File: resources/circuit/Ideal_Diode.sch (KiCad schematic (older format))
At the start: 4 parts, among them Q1 BSS138, U5 DMMT5401

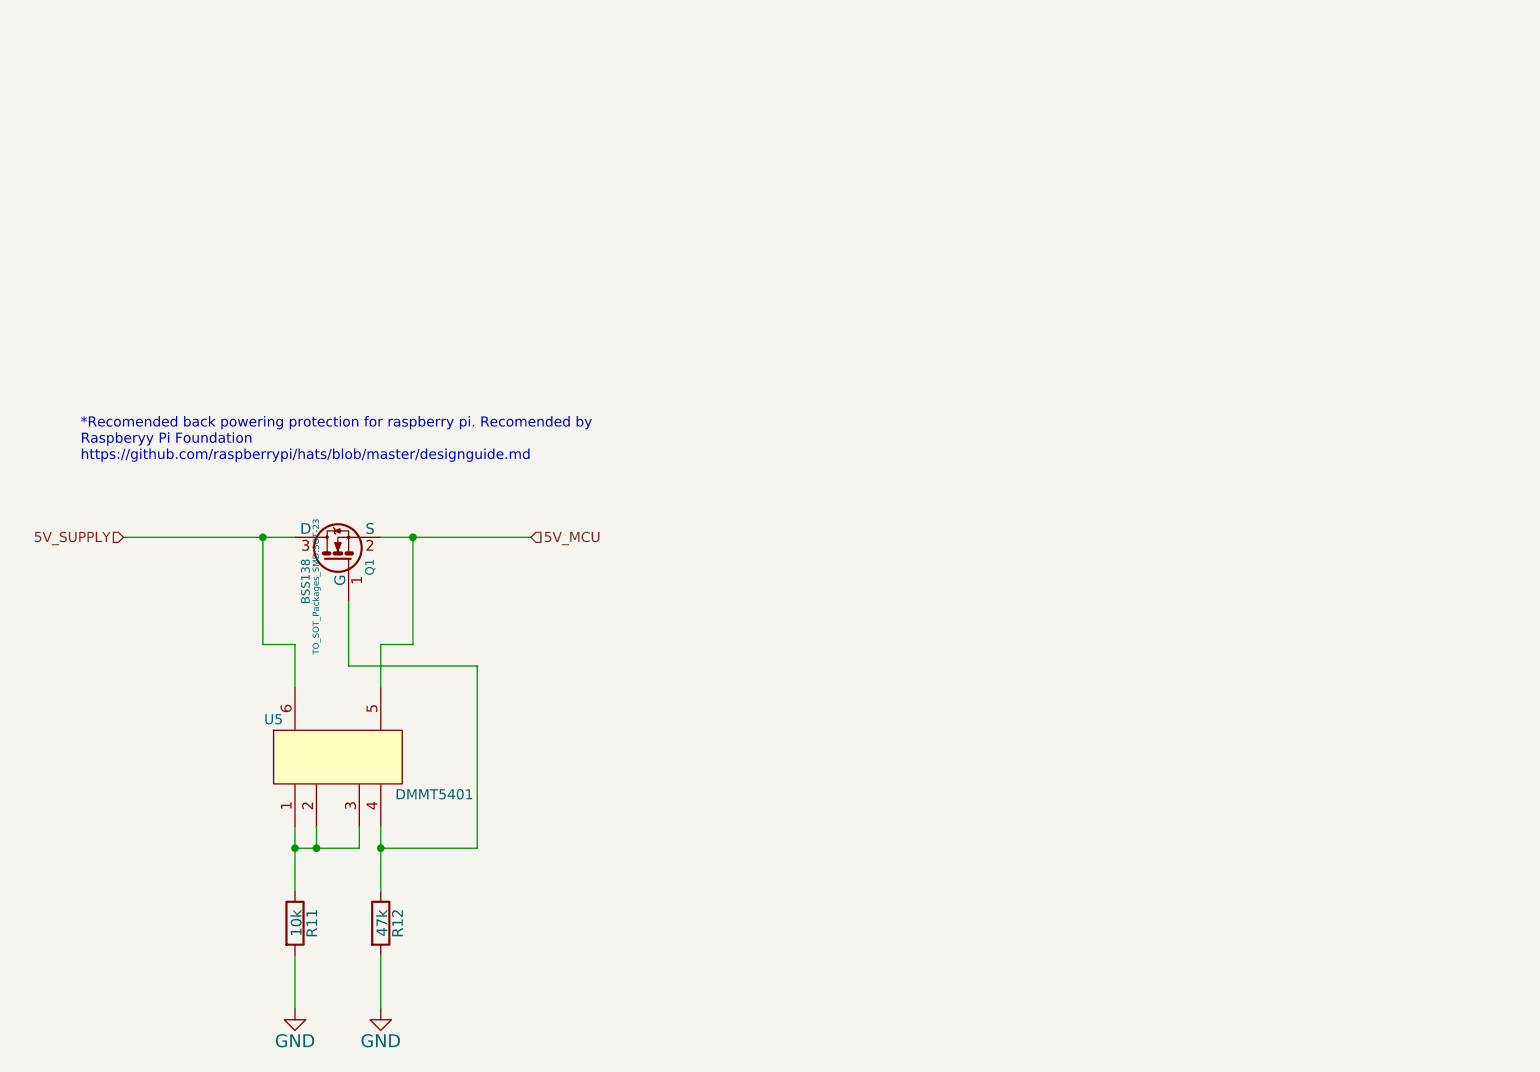
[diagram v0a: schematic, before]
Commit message: Work on circuit & PCB
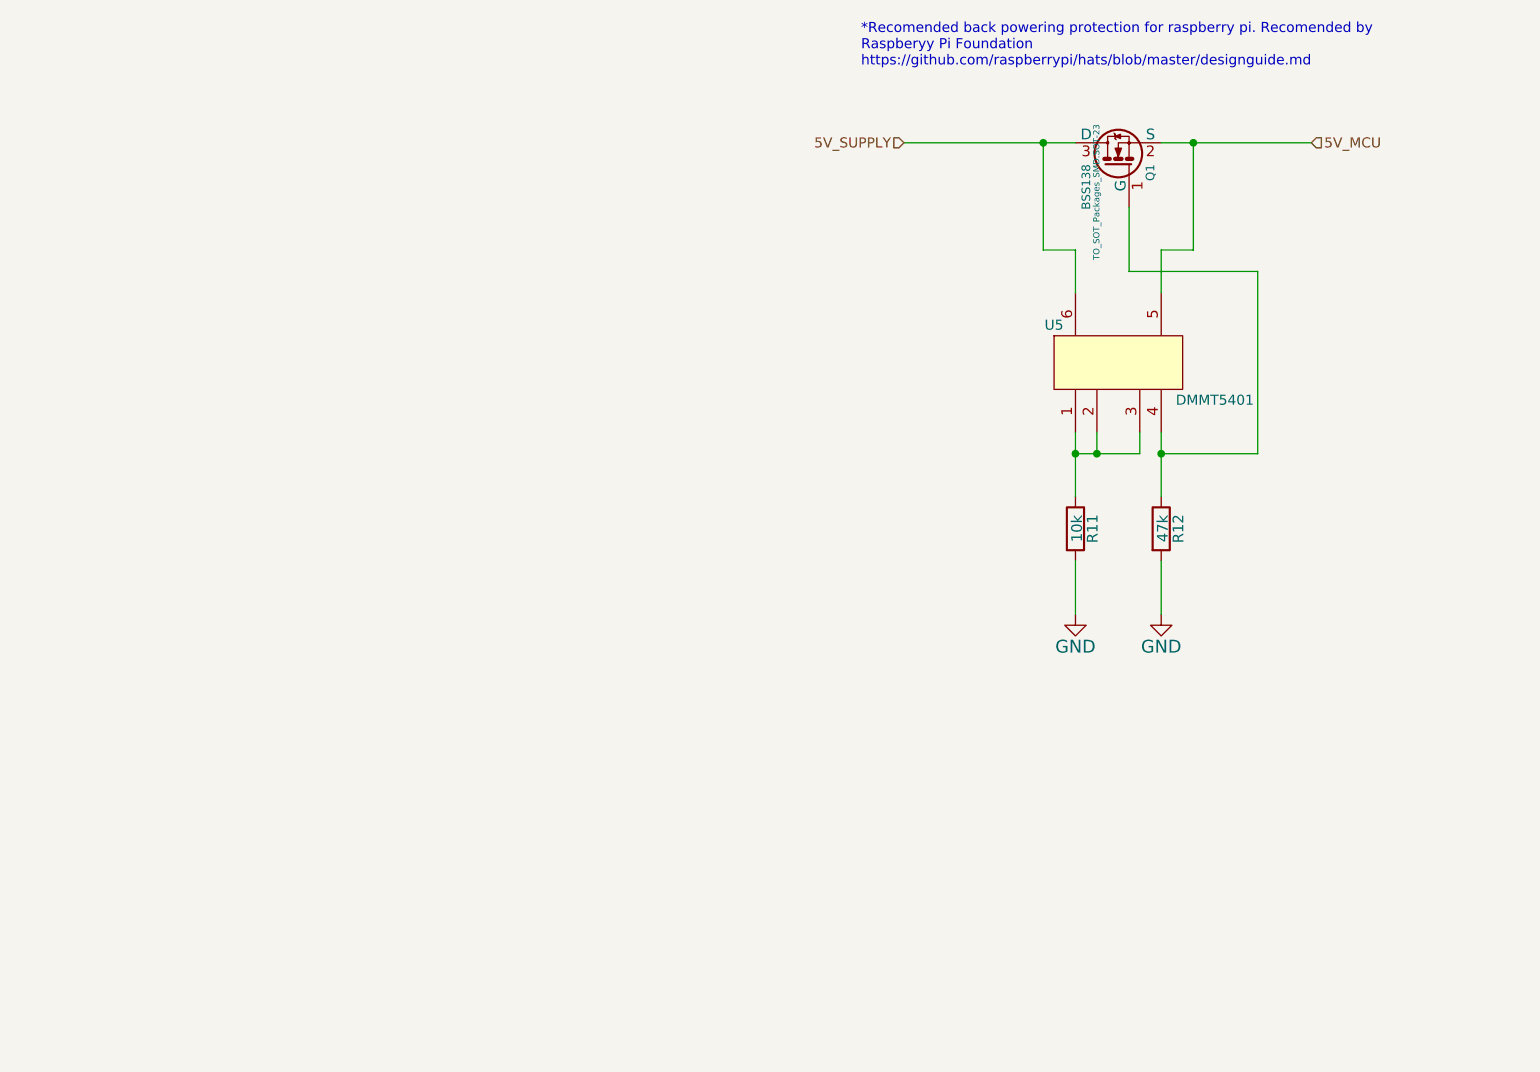
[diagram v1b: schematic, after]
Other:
- moved on the sheet: Q1, R11, R12, U5
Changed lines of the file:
@@
 LIBS:valves
 LIBS:aeroPi
+LIBS:bme280
 LIBS:aeroPi-cache
 EELAYER 25 0
@@
 $Descr A4 11693 8268
 encoding utf-8
-Sheet 2 3
+Sheet 2 2
 Title ""
 Date ""
@@
 L BSS138 Q1
 U 1 1 54F14605
-P 6000 3100
-F 0 "Q1" H 6000 2951 40  0000 R CNN
-F 1 "BSS138" H 6000 3250 40  0000 R CNN
-F 2 "TO_SOT_Packages_SMD:SOT-23" H 5870 3202 29  0000 C CNN
-F 3 "" H 6000 3100 60  0000 C CNN
-F 4 "621-DMG2305UX-13" H 6000 3100 60  0001 C CNN "Mouser Part No."
-	1    6000 3100
+P 9640 1260
+F 0 "Q1" H 9640 1111 40  0000 R CNN
+F 1 "BSS138" H 9640 1410 40  0000 R CNN
+F 2 "TO_SOT_Packages_SMD:SOT-23" H 9510 1362 29  0000 C CNN
+F 3 "" H 9640 1260 60  0000 C CNN
+F 4 "621-DMG2305UX-13" H 9640 1260 60  0001 C CNN "Mouser Part No."
+	1    9640 1260
 	0    -1   -1   0
 $EndComp
-Text HLabel 5000 3000 0    47   Input ~ 0
+Text HLabel 8640 1160 0    47   Input ~ 0
 5V_SUPPLY
-Text HLabel 6900 3000 2    47   Input ~ 0
+Text HLabel 10540 1160 2    47   Input ~ 0
 5V_MCU
 $Comp
 L DMMT5401 U5
 U 1 1 54F1CFA3
-P 6000 4000
-F 0 "U5" H 5700 4150 47  0000 C CNN
-F 1 "DMMT5401" H 6450 3800 47  0000 C CNN
-F 2 "w_smd_trans:sot23-6" H 5850 3700 47  0001 C CNN
-F 3 "" H 5850 3700 47  0000 C CNN
-F 4 "621-DMMT5401-7-F" H 6000 4000 60  0001 C CNN "Mouser Part No."
-	1    6000 4000
+P 9640 2160
+F 0 "U5" H 9340 2310 47  0000 C CNN
+F 1 "DMMT5401" H 10090 1960 47  0000 C CNN
+F 2 "w_smd_trans:sot23-6" H 9490 1860 47  0001 C CNN
+F 3 "" H 9490 1860 47  0000 C CNN
+F 4 "621-DMMT5401-7-F" H 9640 2160 60  0001 C CNN "Mouser Part No."
+	1    9640 2160
 	1    0    0    -1
 $EndComp
 Wire Wire Line
-	6200 3000 6900 3000
+	9840 1160 10540 1160
 Wire Wire Line
-	5000 3000 5800 3000
+	8640 1160 9440 1160
 Wire Wire Line
-	5800 3700 5800 3500
+	9440 1860 9440 1660
 Wire Wire Line
-	5800 3500 5650 3500
+	9440 1660 9290 1660
 Wire Wire Line
-	5650 3500 5650 3000
-Connection ~ 5650 3000
+	9290 1660 9290 1160
+Connection ~ 9290 1160
 Wire Wire Line
-	6200 3700 6200 3500
+	9840 1860 9840 1660
 Wire Wire Line
-	6200 3500 6350 3500
+	9840 1660 9990 1660
 Wire Wire Line
-	6350 3500 6350 3000
-Connection ~ 6350 3000
+	9990 1660 9990 1160
+Connection ~ 9990 1160
 $Comp
 L R R12
 U 1 1 54F1D101
-P 6200 4800
-F 0 "R12" V 6280 4800 50  0000 C CNN
-F 1 "47k" V 6207 4801 50  0000 C CNN
-F 2 "Resistors_SMD:R_0603" V 6130 4800 30  0001 C CNN
-F 3 "" H 6200 4800 30  0000 C CNN
-F 4 "667-ERJ-2RKF4702X" V 6200 4800 60  0001 C CNN "Mouser Part No."
-	1    6200 4800
+P 9840 2960
+F 0 "R12" V 9920 2960 50  0000 C CNN
+F 1 "47k" V 9847 2961 50  0000 C CNN
+F 2 "Resistors_SMD:R_0603" V 9770 2960 30  0001 C CNN
+F 3 "" H 9840 2960 30  0000 C CNN
+F 4 "667-ERJ-2RKF4702X" V 9840 2960 60  0001 C CNN "Mouser Part No."
+	1    9840 2960
 	1    0    0    -1
 $EndComp
@@
 L R R11
 U 1 1 54F1D193
-P 5800 4800
-F 0 "R11" V 5880 4800 50  0000 C CNN
-F 1 "10k" V 5807 4801 50  0000 C CNN
-F 2 "Resistors_SMD:R_0603" V 5730 4800 30  0001 C CNN
-F 3 "" H 5800 4800 30  0000 C CNN
-F 4 "71-CRCW0402-10K-E3" V 5800 4800 60  0001 C CNN "Mouser Part No."
-	1    5800 4800
+P 9440 2960
+F 0 "R11" V 9520 2960 50  0000 C CNN
+F 1 "10k" V 9447 2961 50  0000 C CNN
+F 2 "Resistors_SMD:R_0603" V 9370 2960 30  0001 C CNN
+F 3 "" H 9440 2960 30  0000 C CNN
+F 4 "71-CRCW0402-10K-E3" V 9440 2960 60  0001 C CNN "Mouser Part No."
+	1    9440 2960
 	1    0    0    -1
 $EndComp
@@
 L GND #PWR034
 U 1 1 54F1D1B9
-P 6200 5200
+P 9840 3360
 AR Path="/54F1D1B9" Ref="#PWR034"  Part="1"
-AR Path="/54F145DC/54F1D1B9" Ref="#PWR031"  Part="1"
-F 0 "#PWR031" H 6200 4950 60  0001 C CNN
-F 1 "GND" H 6200 5050 60  0000 C CNN
-F 2 "" H 6200 5200 60  0000 C CNN
-F 3 "" H 6200 5200 60  0000 C CNN
-	1    6200 5200
+AR Path="/54F145DC/54F1D1B9" Ref="#PWR036"  Part="1"
+F 0 "#PWR036" H 9840 3110 60  0001 C CNN
+F 1 "GND" H 9840 3210 60  0000 C CNN
+F 2 "" H 9840 3360 60  0000 C CNN
+F 3 "" H 9840 3360 60  0000 C CNN
+	1    9840 3360
 	1    0    0    -1
 $EndComp
@@
 L GND #PWR035
 U 1 1 54F1D1D3
-P 5800 5200
+P 9440 3360
 AR Path="/54F1D1D3" Ref="#PWR035"  Part="1"
-AR Path="/54F145DC/54F1D1D3" Ref="#PWR032"  Part="1"
-F 0 "#PWR032" H 5800 4950 60  0001 C CNN
-F 1 "GND" H 5800 5050 60  0000 C CNN
-F 2 "" H 5800 5200 60  0000 C CNN
-F 3 "" H 5800 5200 60  0000 C CNN
-	1    5800 5200
+AR Path="/54F145DC/54F1D1D3" Ref="#PWR037"  Part="1"
+F 0 "#PWR037" H 9440 3110 60  0001 C CNN
+F 1 "GND" H 9440 3210 60  0000 C CNN
+F 2 "" H 9440 3360 60  0000 C CNN
+F 3 "" H 9440 3360 60  0000 C CNN
+	1    9440 3360
 	1    0    0    -1
 $EndComp
 Wire Wire Line
-	5800 4350 5800 4650
+	9440 2510 9440 2810
 Wire Wire Line
-	5800 4950 5800 5200
+	9440 3110 9440 3360
 Wire Wire Line
-	6200 4350 6200 4650
+	9840 2510 9840 2810
 Wire Wire Line
-	6200 4950 6200 5200
+	9840 3110 9840 3360
 Wire Wire Line
-	5900 4350 5900 4450
+	9540 2510 9540 2610
 Wire Wire Line
-	5800 4450 6100 4450
-Connection ~ 5800 4450
+	9440 2610 9740 2610
+Connection ~ 9440 2610
 Wire Wire Line
-	6100 4450 6100 4350
-Connection ~ 5900 4450
+	9740 2610 9740 2510
+Connection ~ 9540 2610
 Wire Wire Line
-	6050 3300 6050 3600
+	9690 1460 9690 1760
 Wire Wire Line
-	6050 3600 6650 3600
+	9690 1760 10290 1760
 Wire Wire Line
-	6650 3600 6650 4450
+	10290 1760 10290 2610
 Wire Wire Line
-	6650 4450 6200 4450
-Connection ~ 6200 4450
-Text Notes 4800 2650 0    47   ~ 0
+	10290 2610 9840 2610
+Connection ~ 9840 2610
+Text Notes 8440 810  0    47   ~ 0
 *Recomended back powering protection for raspberry pi. Recomended by\nRaspberyy Pi Foundation\nhttps://github.com/raspberrypi/hats/blob/master/designguide.md
 $EndSCHEMATC

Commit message: Work on circuit and add documentation + 3D model
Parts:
- Q1: symbol BSS138 -> BSS138-RESCUE-aeroPi
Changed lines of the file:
@@
 EESchema Schematic File Version 2
+LIBS:aeroPi-rescue
 LIBS:power
 LIBS:device
@@
 $EndDescr
 $Comp
-L BSS138 Q1
+L BSS138-RESCUE-aeroPi Q1
 U 1 1 54F14605
 P 9640 1260
@@
 P 9840 3360
 AR Path="/54F1D1B9" Ref="#PWR034"  Part="1"
-AR Path="/54F145DC/54F1D1B9" Ref="#PWR036"  Part="1"
-F 0 "#PWR036" H 9840 3110 60  0001 C CNN
+AR Path="/54F145DC/54F1D1B9" Ref="#PWR038"  Part="1"
+F 0 "#PWR038" H 9840 3110 60  0001 C CNN
 F 1 "GND" H 9840 3210 60  0000 C CNN
 F 2 "" H 9840 3360 60  0000 C CNN
@@
 P 9440 3360
 AR Path="/54F1D1D3" Ref="#PWR035"  Part="1"
-AR Path="/54F145DC/54F1D1D3" Ref="#PWR037"  Part="1"
-F 0 "#PWR037" H 9440 3110 60  0001 C CNN
+AR Path="/54F145DC/54F1D1D3" Ref="#PWR039"  Part="1"
+F 0 "#PWR039" H 9440 3110 60  0001 C CNN
 F 1 "GND" H 9440 3210 60  0000 C CNN
 F 2 "" H 9440 3360 60  0000 C CNN
